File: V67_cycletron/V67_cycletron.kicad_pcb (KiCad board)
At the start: 2 copper layers, 99 x 101 mm, 41 parts, among them J1 USB_C_Receptacle_USB2.0_16P, J2 Screw_Terminal_01x02, J3 Screw_Terminal_01x14, J4 Screw_Terminal_01x02, U1 ESP32-S3-WROOM-1, U2 LM1117DT-3.3, U3 LM1117DT-5.0

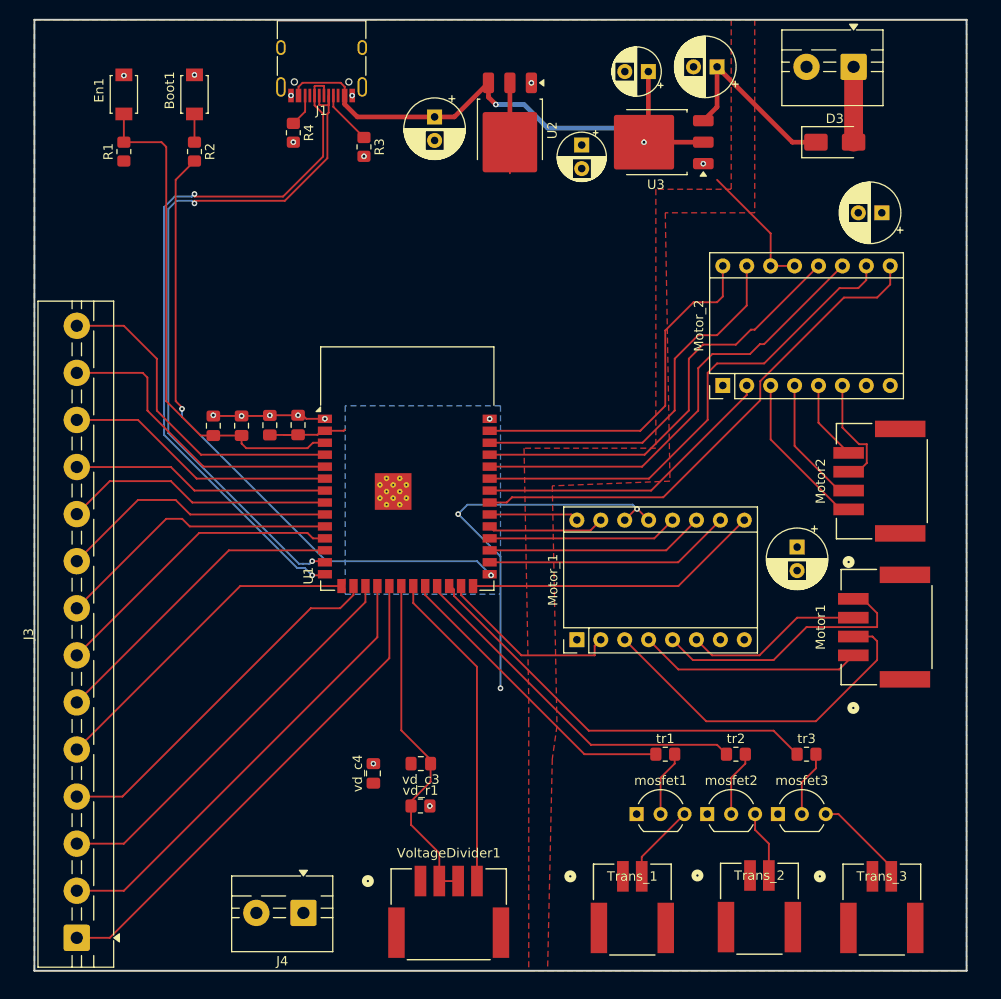
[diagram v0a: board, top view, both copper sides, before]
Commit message: got all parts to sync to jlcpcb
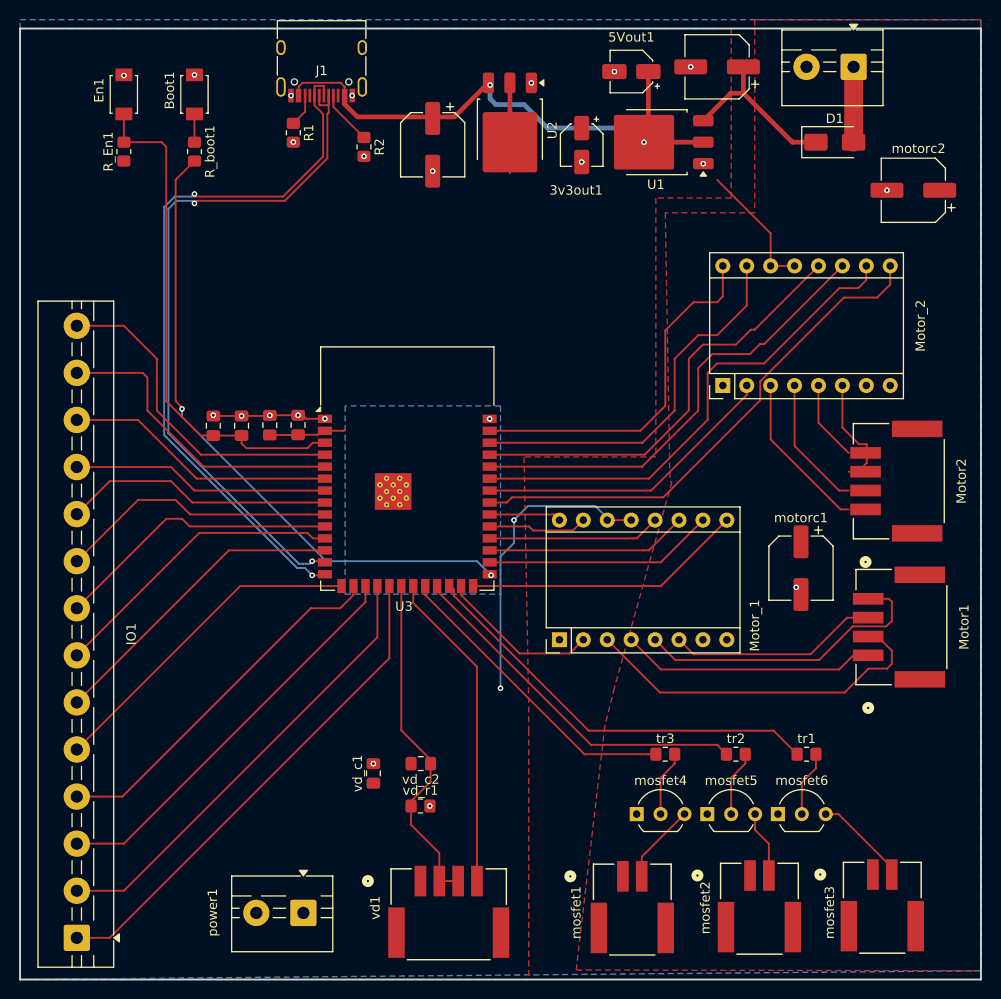
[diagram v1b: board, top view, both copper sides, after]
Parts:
- removed Trans_3: 5023520200, Connector_4:CONN_SD-502352-001_02_MOL
- added mosfet3: 5023520200, Connector_4:CONN_SD-502352-001_02_MOL, F.Cu at (193.5, 114.8)
- 3v3in1: renamed from reg_3v3_smoother_in1; footprint Capacitor_THT:CP_Radial_D6.3mm_P2.50mm -> Capacitor_SMD:CP_Elec_6.3x5.4
- 3v3out1: renamed from reg_3v3_smoother_out1; footprint Capacitor_THT:CP_Radial_D5.0mm_P2.50mm -> Capacitor_SMD:CP_Elec_4x5.4
- 5Vin1: renamed from reg_5V_smoothing_caps_in1; footprint Capacitor_THT:CP_Radial_D6.3mm_P2.50mm -> Capacitor_SMD:CP_Elec_6.3x5.4
- 5Vout1: renamed from reg_5V_smoothing_caps_out1; footprint Capacitor_THT:CP_Radial_D5.0mm_P2.50mm -> Capacitor_SMD:CP_Elec_4x5.4
- motorc1: renamed from motor1_c1; value C_Polarized -> 100uF; footprint Capacitor_THT:CP_Radial_D6.3mm_P2.50mm -> Capacitor_SMD:CP_Elec_6.3x5.4
- motorc2: renamed from motor2_c1; value C_Polarized -> 100uF; footprint Capacitor_THT:CP_Radial_D6.3mm_P2.50mm -> Capacitor_SMD:CP_Elec_6.3x5.4
- moved motorc2 4.11 mm to (196.8, 38.6)
- moved 3v3in1 2.97 mm to (145.8, 33.8)
- moved motorc1 2.28 mm to (184.9, 78.7)
- moved Motor_1 1.85 mm to (159.3, 86.3)
- moved 5Vout1 1.81 mm to (166.9, 26.0)
- moved Motor2 1.80 mm to (195.3, 69.5)
- moved Motor1 1.58 mm to (195.6, 85.0)
- renumbered C6 to C1, C8 to C2, D3 to D1, J3 to IO1, R4 to R1, R3 to R2, R1 to R_En1, R2 to R_boot1, U3 to U1, U1 to U3, J2 to input1, Trans_1 to mosfet1, Trans_2 to mosfet2, mosfet1 to mosfet4, mosfet2 to mosfet5, mosfet3 to mosfet6, J4 to power1, esp_smoothingcaps_1 to smooth_cap1, esp_smoothingcaps_2 to smooth_cap2, tr3 to tr1, tr1 to tr3, VoltageDivider1 to vd1, vd_c4 to vd_c1, vd_c3 to vd_c2
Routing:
- net 3V3: track 81.4 -> 70.1 mm
- net Motor1_B1: track 28.7 -> 32.4 mm
- net Motor1_A2: track 37.8 -> 41.1 mm
- net Motor1_FLT: track 19.7 -> 17.1 mm
- net +12V: track 20.1 -> 18.1 mm
- net Motor1_STEP: track 12.4 -> 10.6 mm
- net Motor1_M2: track 20.2 -> 18.4 mm
- net Motor1_M1: track 23.3 -> 21.4 mm
- net Motor1_M0: track 26.4 -> 24.5 mm
- net Motor1_DIR: track 9.51 -> 7.66 mm
- net Motor1_A1: track 23.7 -> 25.5 mm
- net Motor1_EN: track 31.7 -> 29.9 mm
- net Motor1_B2: track 19.0 -> 20.8 mm
- net GND: vias 16 -> 23
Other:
- board size 99 x 101 mm -> 102 x 101 mm
